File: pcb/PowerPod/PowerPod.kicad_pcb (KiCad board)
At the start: 4 copper layers, 47 x 40 mm, 67 parts, among them IC2 FUSB302MPX, IC3 CC6904SO-10A, IC4 TPS62175DQCT, IC5 ESP32-C3FH4, J1 GT-USB-7010, J2 TC2050-IDC, J3 KF350-3.5-2P, J5 Conn_01x06, U1 SRV05-4, Y2 SX25Y040000BF1T-C

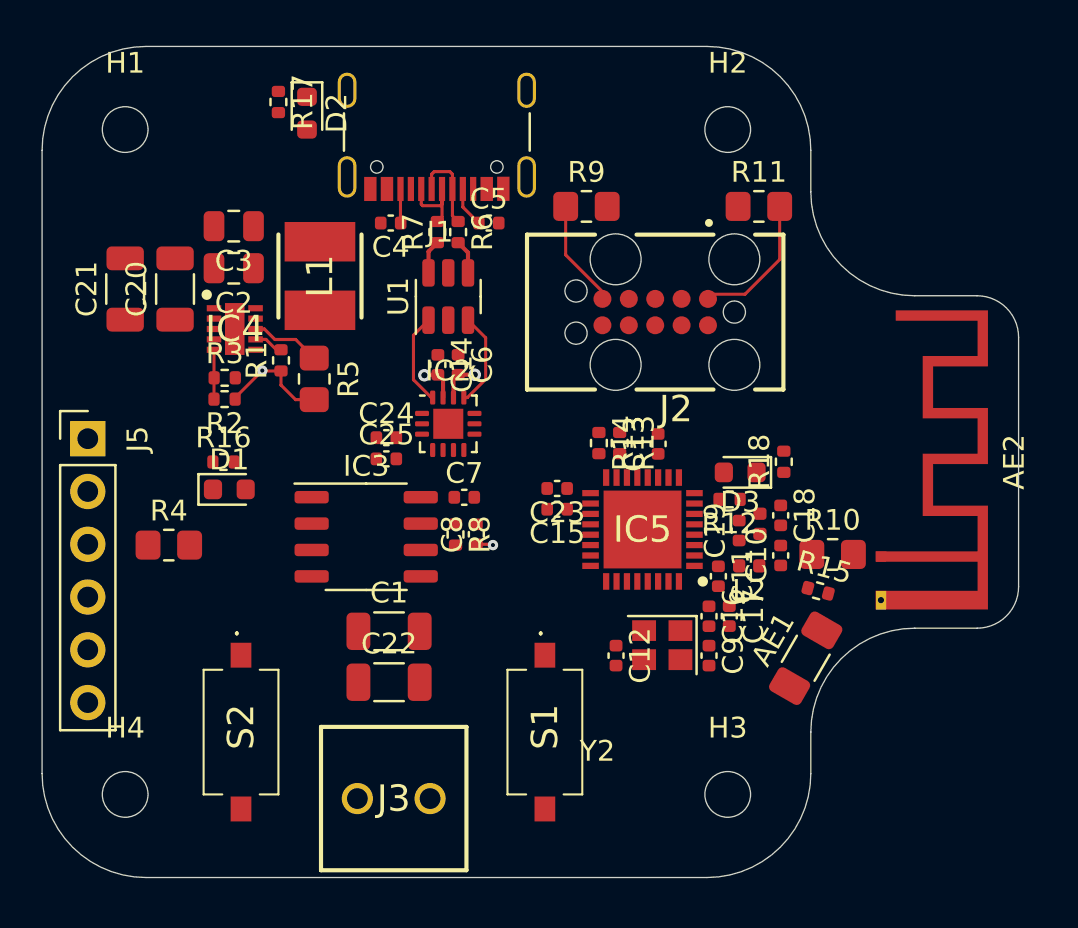
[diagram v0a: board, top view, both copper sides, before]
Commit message: finished layout
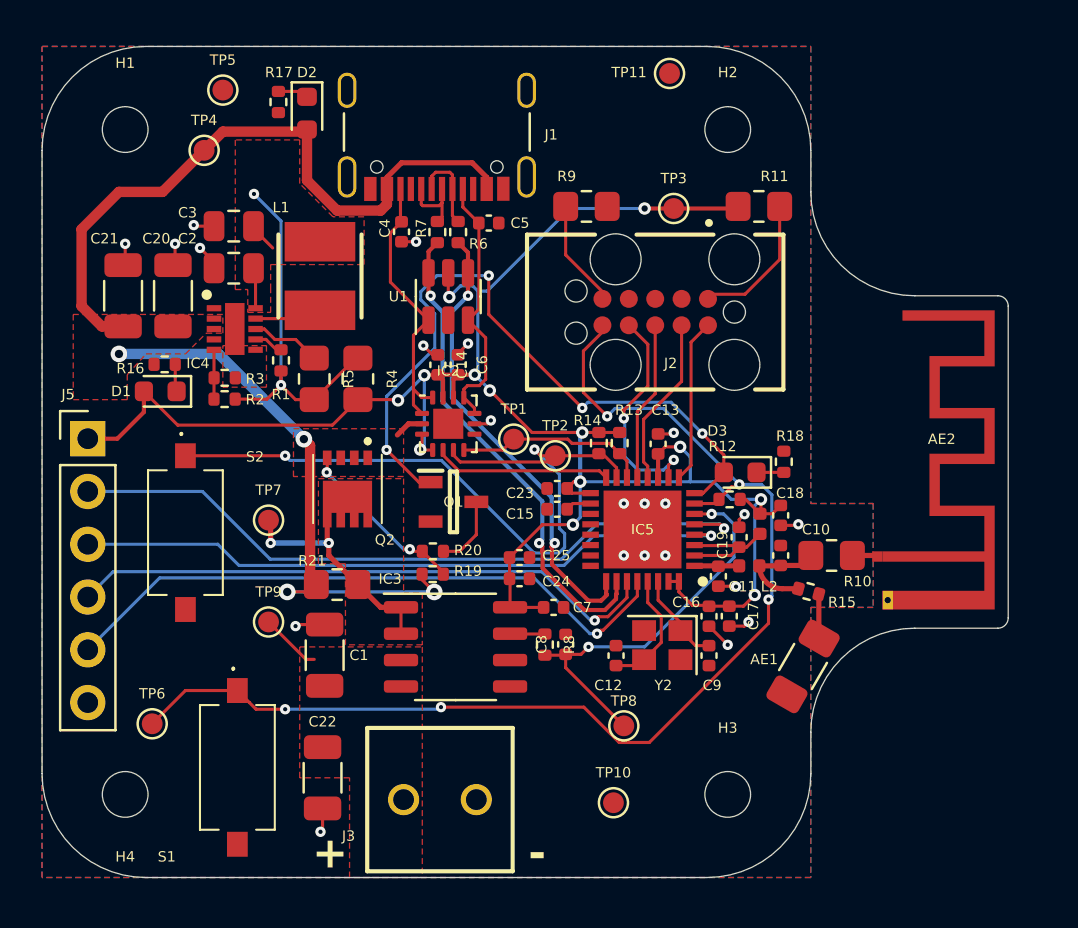
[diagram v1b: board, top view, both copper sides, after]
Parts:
- added Q1: DTC143ECA-TP, SamacSys_Parts:SOT95P237X125-3N, F.Cu at (197.8, 121.9)
- added Q2: DMP3017SFG-7, SamacSys_Parts:DMP3007SFG7, F.Cu at (192.7, 121.3)
- added R19: 10k, Resistor_SMD:R_0402_1005Metric, F.Cu at (196.8, 125.4)
- added R20: 1k, Resistor_SMD:R_0402_1005Metric, F.Cu at (196.8, 124.3)
- added R21: DNF_0805, Resistor_SMD:R_0805_2012Metric_Pad1.20x1.40mm_HandSolder, F.Cu at (192.2, 125.9)
- added TP1: TestPoint, TestPoint:TestPoint_Pad_D1.0mm, F.Cu at (200.7, 118.9)
- added TP10: TestPoint, TestPoint:TestPoint_Pad_D1.0mm, F.Cu at (205.5, 136.4)
- added TP11: TestPoint, TestPoint:TestPoint_Pad_D1.0mm, F.Cu at (208.2, 101.3)
- added TP2: TestPoint, TestPoint:TestPoint_Pad_D1.0mm, F.Cu at (202.7, 119.7)
- added TP3: TestPoint, TestPoint:TestPoint_Pad_D1.0mm, F.Cu at (208.4, 107.8)
- added TP4: TestPoint, TestPoint:TestPoint_Pad_D1.0mm, F.Cu at (185.8, 105.0)
- added TP5: TestPoint, TestPoint:TestPoint_Pad_D1.0mm, F.Cu at (186.7, 102.1)
- added TP6: TestPoint, TestPoint:TestPoint_Pad_D1.0mm, F.Cu at (183.3, 132.6)
- added TP7: TestPoint, TestPoint:TestPoint_Pad_D1.0mm, F.Cu at (188.9, 122.8)
- added TP8: TestPoint, TestPoint:TestPoint_Pad_D1.0mm, F.Cu at (206.0, 132.7)
- added TP9: TestPoint, TestPoint:TestPoint_Pad_D1.0mm, F.Cu at (188.9, 127.7)
- moved S1 14.9 mm to (187.4, 134.7)
- moved R4 12.1 mm to (193.2, 116.0), turned to -90 degrees
- moved S2 9.97 mm to (184.9, 123.4)
- moved C24 9.34 mm to (201.0, 125.6), turned to 180 degrees
- moved C25 7.98 mm to (201.0, 124.6), turned to 180 degrees
- moved IC3 6.82 mm to (197.9, 128.9)
- moved C7 6.82 mm to (202.6, 127.0)
- moved C8 6.82 mm to (203.2, 128.8)
- moved R8 6.82 mm to (202.2, 128.8)
- moved D1 5.77 mm to (183.7, 116.6), turned to 180 degrees
- moved C22 5.60 mm to (191.5, 135.2), turned to -90 degrees
- moved R16 5.49 mm to (183.9, 115.3), turned to 180 degrees
- moved C1 3.31 mm to (191.6, 129.3), turned to 90 degrees
- moved J3 2.23 mm to (195.4, 136.2)
- moved C4 0.67 mm to (195.3, 108.9), turned to -90 degrees
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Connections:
- net /Current Sensor/VOUT renamed /Current Sensor + Output Control/VOUT
- net /Current Sensor/V_CURRENT renamed /Current Sensor + Output Control/V_CURRENT
- IC3 pad 1: VBUS -> Net-(Q2-D_1)
- IC3 pad 2: VBUS -> Net-(Q2-D_1)
- J5 pad 2: /Microcontroller/U0RXD -> /Microcontroller/GPIO1
- J5 pad 3: /Microcontroller/U0TXD -> /Microcontroller/GPIO0
- J5 pad 4: /Microcontroller/GPIO0 -> /Microcontroller/U0RXD
- J5 pad 5: /Microcontroller/GPIO1 -> /Microcontroller/U0TXD
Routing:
- net +3V3: track 3.85 -> 98.9 mm, vias 2 -> 13
- net VBUS: track 0.00 -> 61.1 mm, vias 0 -> 4
- net /Microcontroller/EN: track 0.00 -> 57.3 mm, vias 0 -> 5
- net /Microcontroller/GPIO9: track 0.00 -> 35.3 mm, vias 0 -> 2
- net /Microcontroller/GPIO1: track 0.00 -> 34.3 mm, vias 0 -> 1
- net /Microcontroller/GPIO3: track 0.00 -> 34.1 mm, vias 0 -> 4
- net /Microcontroller/GPIO0: track 0.00 -> 31.8 mm, vias 0 -> 1
- net /Microcontroller/U0TXD: track 0.00 -> 30.4 mm, vias 0 -> 1
- net /Microcontroller/U0RXD: track 0.00 -> 28.7 mm, vias 0 -> 1
- net /Microcontroller/USB_DP: track 1.63 -> 23.7 mm, vias 0 -> 2
- net /Microcontroller/USB_DN: track 1.65 -> 22.3 mm, vias 0 -> 2
- net /Current Sensor + Output Control/V_CURRENT: track 0.82 -> 19.3 mm, vias 1 -> 2
- net Net-(IC4-VOS): track 5.39 -> 20.8 mm, vias 1 -> 2
- net GND: track 0.00 -> 15.2 mm, vias 0 -> 22
- net Net-(Q2-D_1): track 0.00 -> 11.3 mm, vias 0 -> 2
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- added copper zone on F.Cu, net /Current Sensor + Output Control/VOUT
- added copper zone on B.Cu, net GND
- added copper zone on F.Cu, net GND
- added copper zone on In1.Cu, net GND
- added copper zone on In2.Cu, net GND
- added copper zone on F.Cu, net Net-(IC4-VOS)
- added copper zone on F.Cu, net Net-(Q2-D_1)
- added copper zone on F.Cu, net VBUS
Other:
- board size 47 x 40 mm -> 46.5 x 40 mm
- board text added: "+"
- board text added: "-"
